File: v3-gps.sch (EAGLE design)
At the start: 199 parts, among them J1 1.27MM-SWD-CONNECTOR, J2 CON_SMA-ENDFIRE_EMERSON_EMERS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, J3 ROCKETNET-CONNECTOR-16M, J4 ZX62D-B-5P8, J7 CON_HIROSE_DM3D(MICROSD), Q1 NTR4101P, T1 ALT4532, T2 ALT4532, U1 MAX2769ETI+, U10 BP2G+, U11 MAX8510EXK29+T, U12 ALM-GP002, U13 XC2C32A_VQ44_2, U14 MIC5319-1.8V, U2 STM32F407VG, U3 KSZ8081, U4 7Q-16.368MBG-T, U5 LT1719S6, U6 MAX8510EXK29+T, U7 MAX8510EXK29+T, U8 LMZ12001TZ-ADJ/NOPB, U9 VENUS638FLPX-L, X1 25 MHz

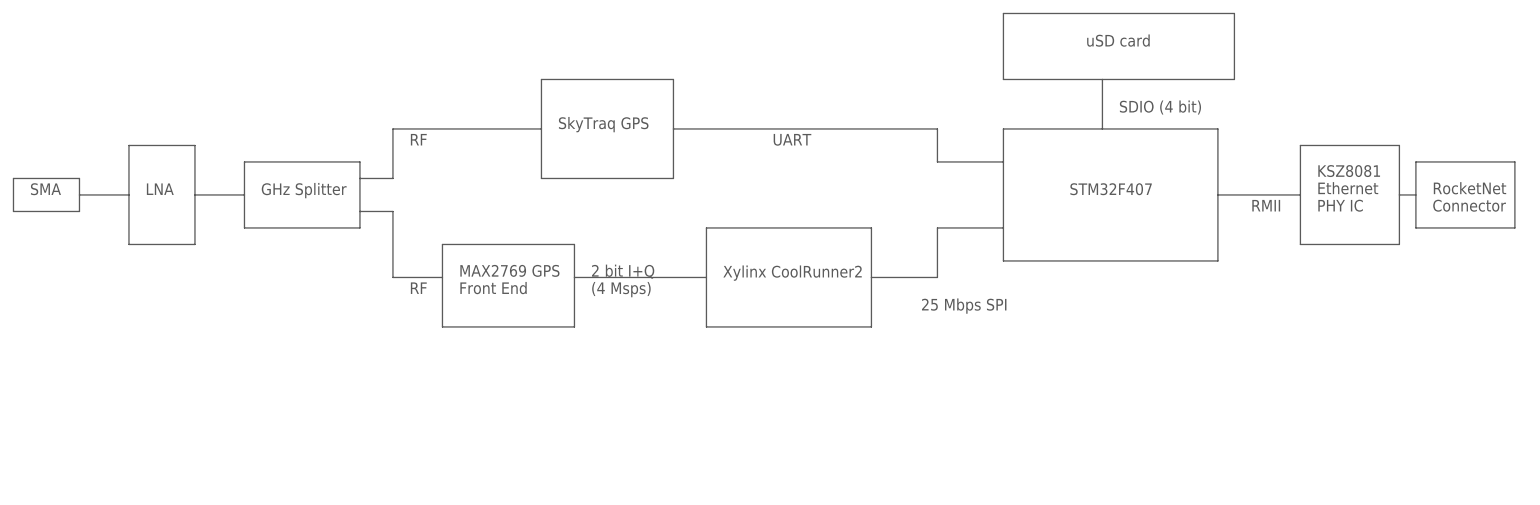
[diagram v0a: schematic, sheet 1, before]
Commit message: OK now it's really done. tnames cleaned up more, ERC and DRC gone over, BOM updated and price calculated, found lack of stock on certain items, etc.
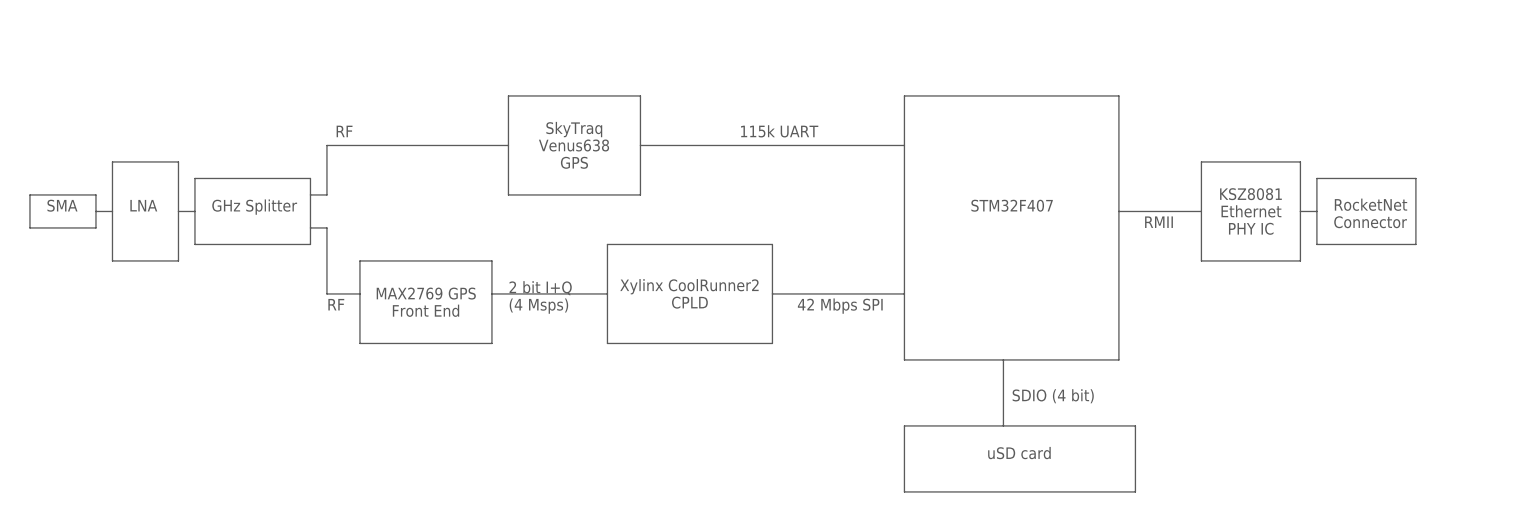
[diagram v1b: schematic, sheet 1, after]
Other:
- note added: "115k UART"
- note added: "42 Mbps SPI"
- note added: "SkyTraq Venus638 GPS"
- note added: "Xylinx CoolRunner2 CPLD"
- note removed: "25 Mbps SPI"
- note removed: "SkyTraq GPS"
- note removed: "UART"
- note removed: "Xylinx CoolRunner2"
